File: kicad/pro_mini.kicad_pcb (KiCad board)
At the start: 2 copper layers, 17.8 x 33 mm, 14 parts, among them IC1 ATMEGA328P-A, P1 FTDI, P2 DIGITAL, P3 CONN_01X12, U1 MCP1700T-3302E

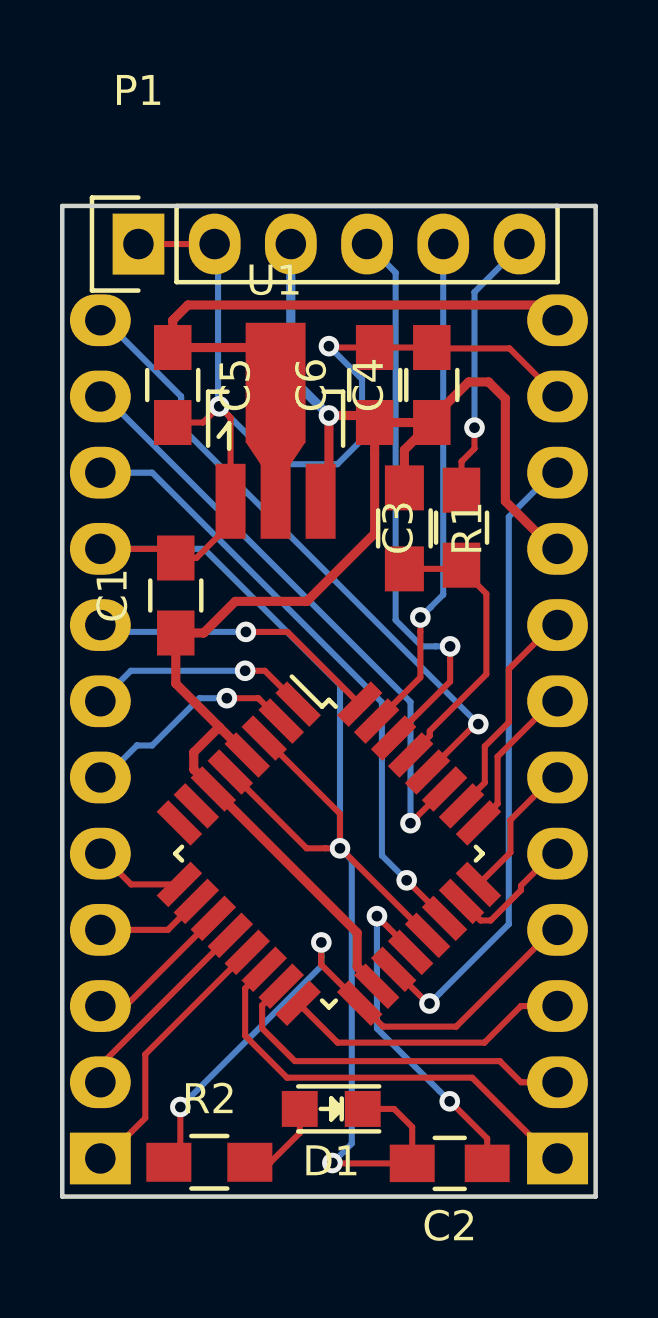
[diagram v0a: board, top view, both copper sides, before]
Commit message: Room for pin labels
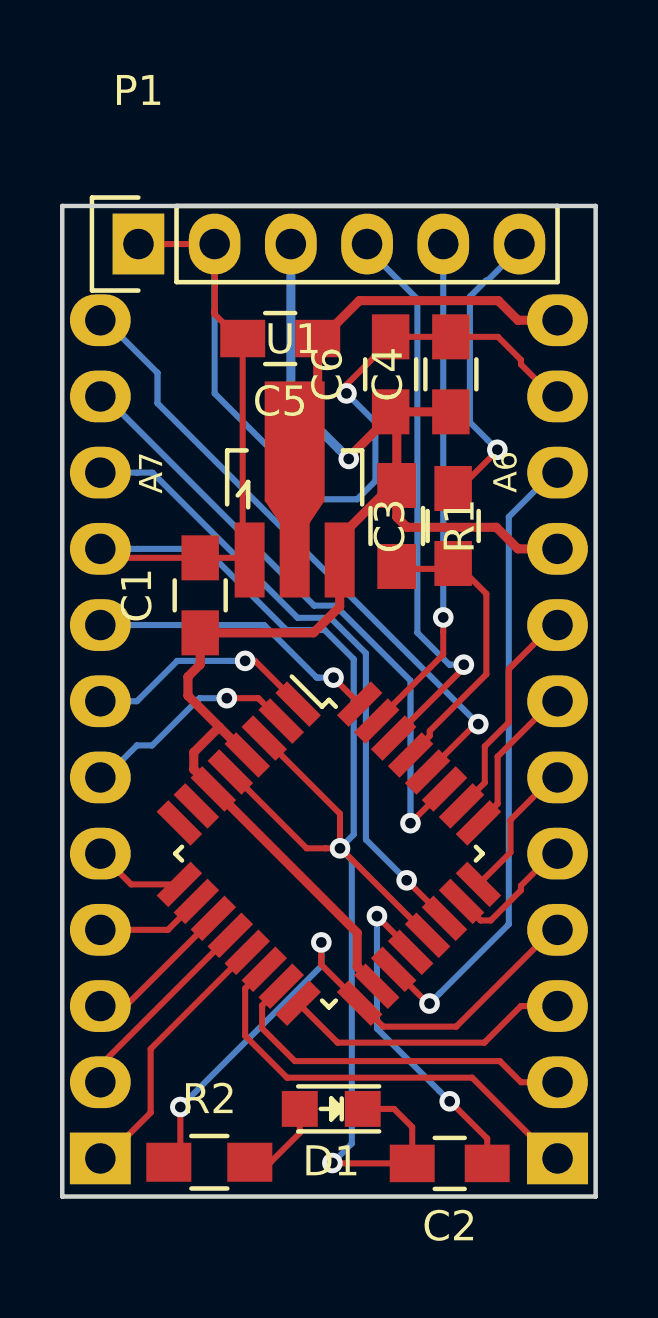
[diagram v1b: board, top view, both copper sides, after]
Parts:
- moved C5 3.90 mm to (108.9, 103.5), turned to 180 degrees
- moved U1 2.06 mm to (109.3, 108.5)
- moved C1 0.81 mm to (106.2, 112.0)
- moved C4 0.73 mm to (114.6, 104.7)
- moved C6 0.64 mm to (112.5, 104.7)
- moved C3 0.28 mm to (114.6, 109.7)
- moved R1 0.27 mm to (112.8, 109.7)
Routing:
- net GND: track 82.3 -> 90.0 mm, vias 4 -> 3
- net RAW: track 24.2 -> 18.8 mm
- net VCC: track 52.9 -> 48.2 mm
- net DTR: track 9.10 -> 9.79 mm
- net A7: track 20.6 -> 21.3 mm
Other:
- board text added: "A6"
- board text added: "A7"
